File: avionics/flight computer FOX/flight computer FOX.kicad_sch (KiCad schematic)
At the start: 21 parts, among them J1 Screw_Terminal_01x02, J2 Conn_01x03, J3 Conn_01x03, J4 Conn_01x03, J5 Conn_01x03, J6 Conn_01x03, U1 ESP32-DevKitC, U2 LM7805_TO220

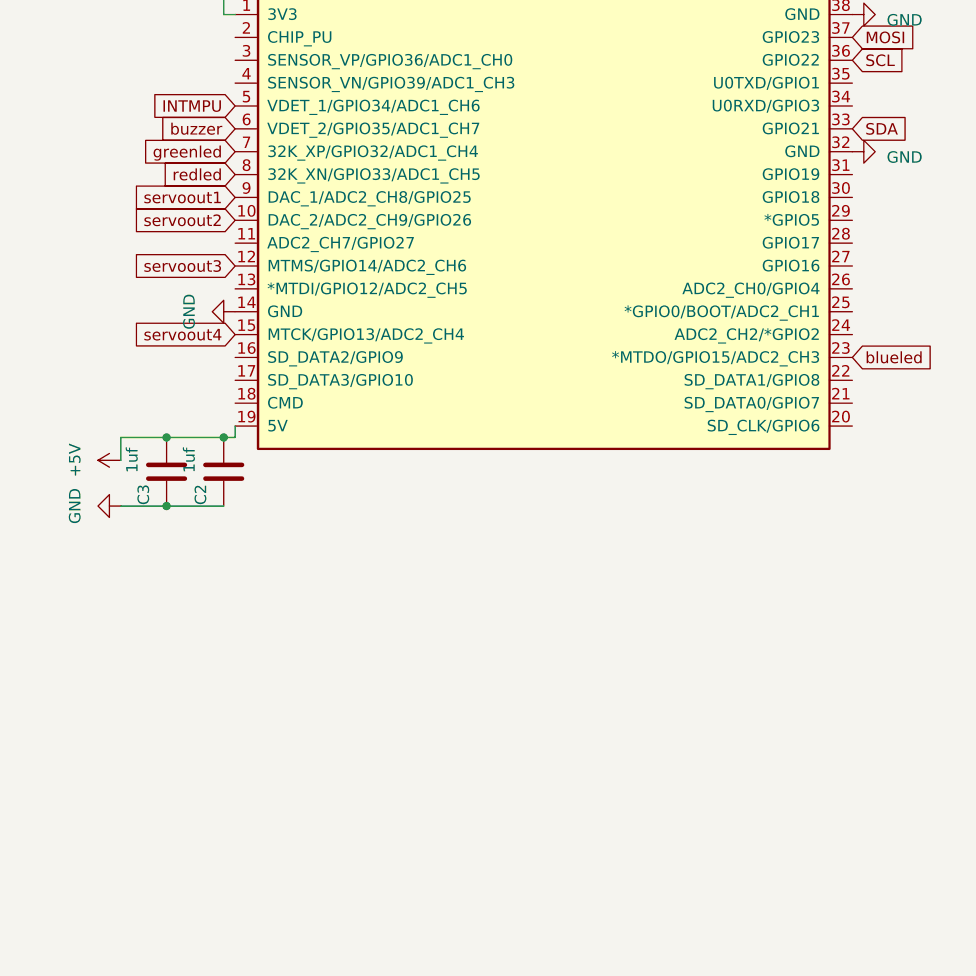
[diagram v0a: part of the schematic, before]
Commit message: more avionics work
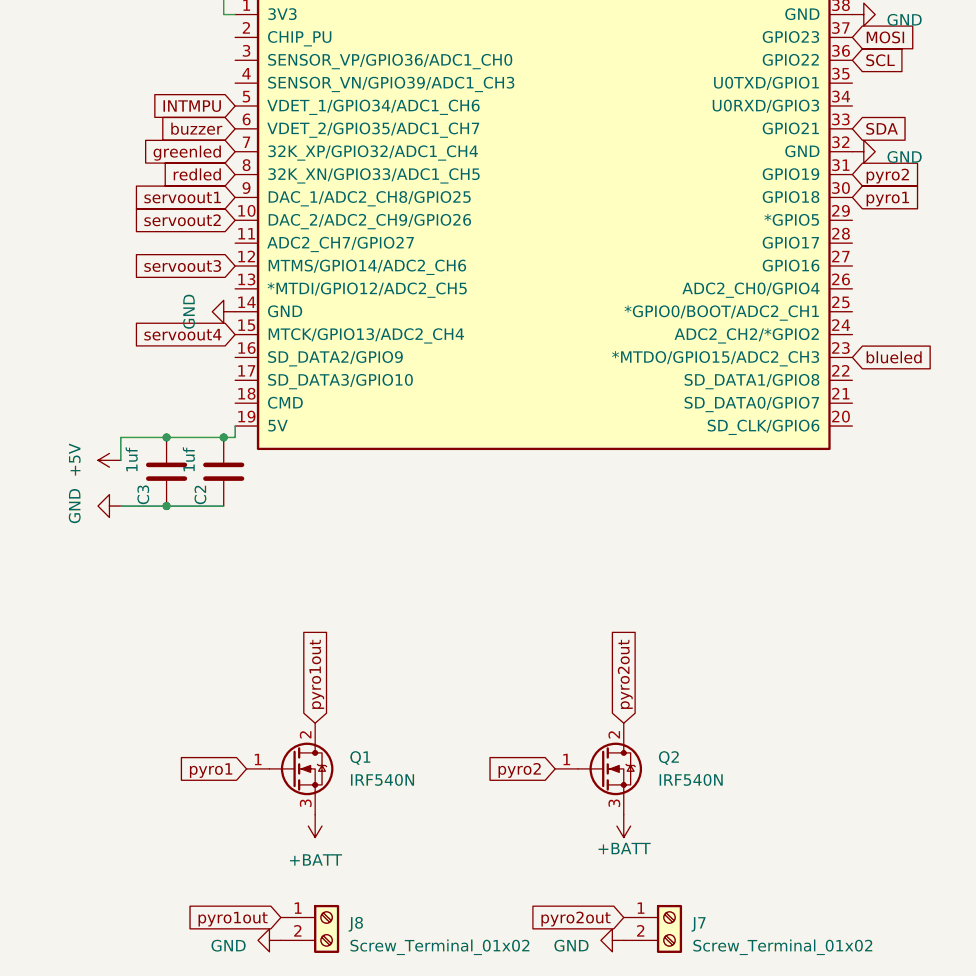
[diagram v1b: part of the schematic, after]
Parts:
- added J7, J8: Screw_Terminal_01x02, TerminalBlock:TerminalBlock_bornier-2_P5.08mm, symbol Connector:Screw_Terminal_01x02
- added Q1, Q2: IRF540N, Package_TO_SOT_THT:TO-220-3_Vertical, symbol Transistor_FET:IRF540N
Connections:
- net +BATT: now also Q1.3 (S), Q2.3 (S)
- net GND: now also J7.2 (Pin_2), J8.2 (Pin_2)
- net pyro1: now reaches U1.30 (GPIO18)
- net pyro1: now also Q1.1 (G)
- net pyro2: now reaches U1.31 (GPIO19)
- net pyro2: now also Q2.1 (G)
- new net pyro1out: J8.1 (Pin_1), Q1.2 (D)
- new net pyro2out: J7.1 (Pin_1), Q2.2 (D)
